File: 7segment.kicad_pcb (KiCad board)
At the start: 4 copper layers, 22.5 x 25.1 mm, 30 parts, among them J1 AVR-ISP-6, J2 Conn_01x10, J4 Conn_01x02, Q1 Q_NPN_BEC, Q2 Q_NPN_BEC, U1 ATmega168PA-AU, U2 HDSP-523

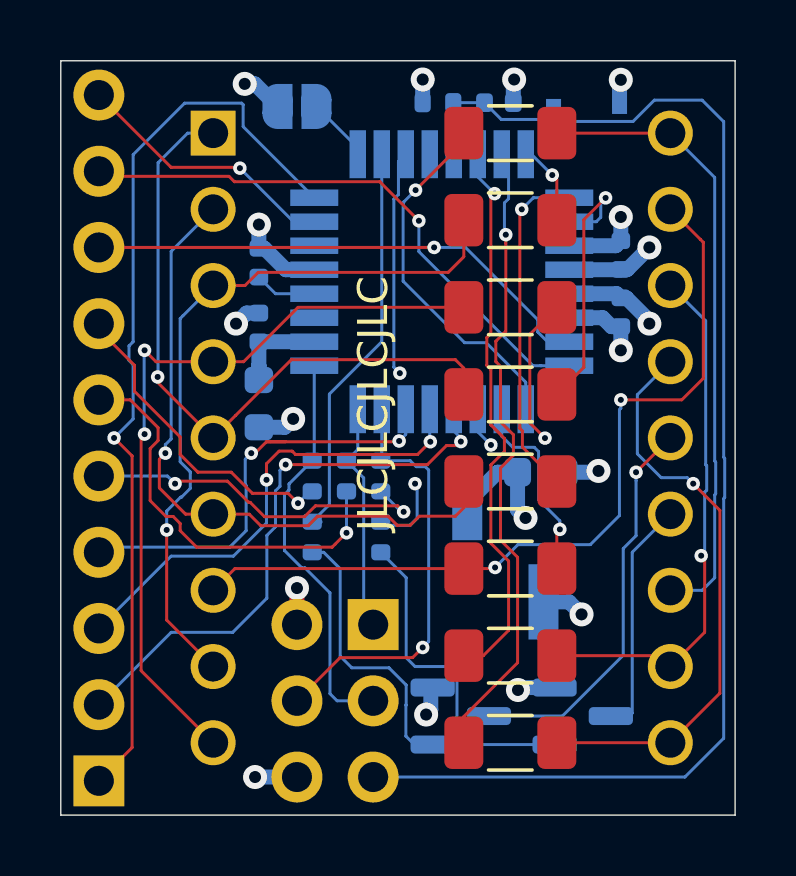
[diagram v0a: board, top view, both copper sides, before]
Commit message: Update
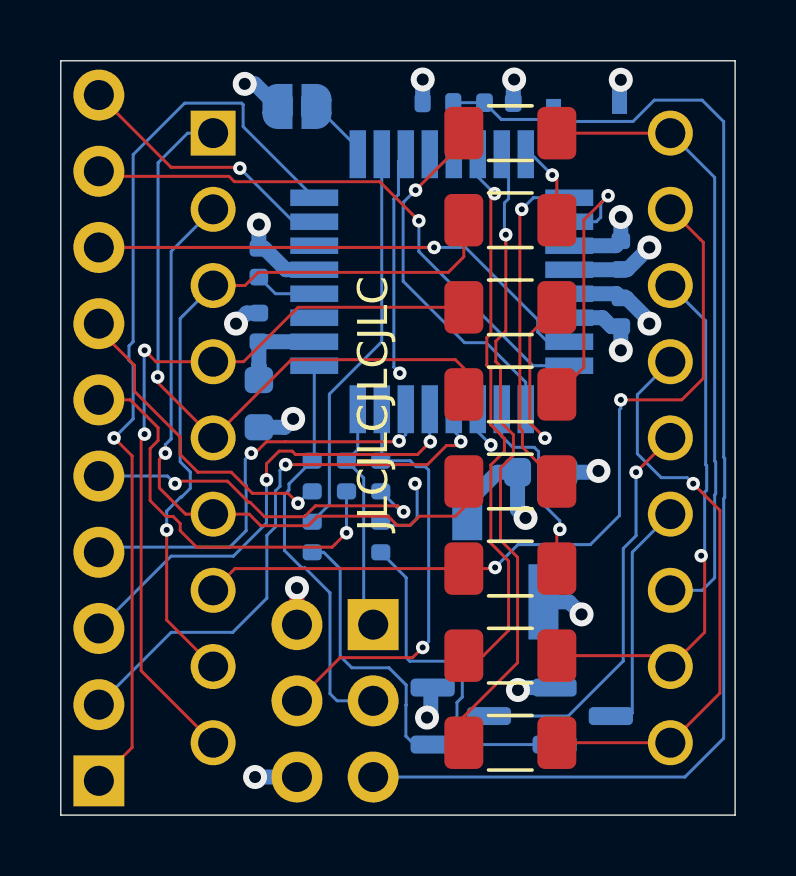
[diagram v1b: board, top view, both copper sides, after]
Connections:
- net +5V renamed VCC
- U1 pad 19: Net-(U1-Pad19) -> unconnected-(U1-Pad19)
- U1 pad 22: Net-(U1-Pad22) -> unconnected-(U1-Pad22)
- U1 pad 28: Net-(U1-Pad28) -> unconnected-(U1-Pad28)
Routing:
- net /D2: track 14.8 -> 14.1 mm

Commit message: Update
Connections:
- net /ZERO_I_OR_LE renamed /ZERO_I_OR_OE
